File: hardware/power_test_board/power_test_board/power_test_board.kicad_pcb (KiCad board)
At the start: 2 copper layers, 21 parts, among them SW1 YTSC005A0152501B, U1 AXP192

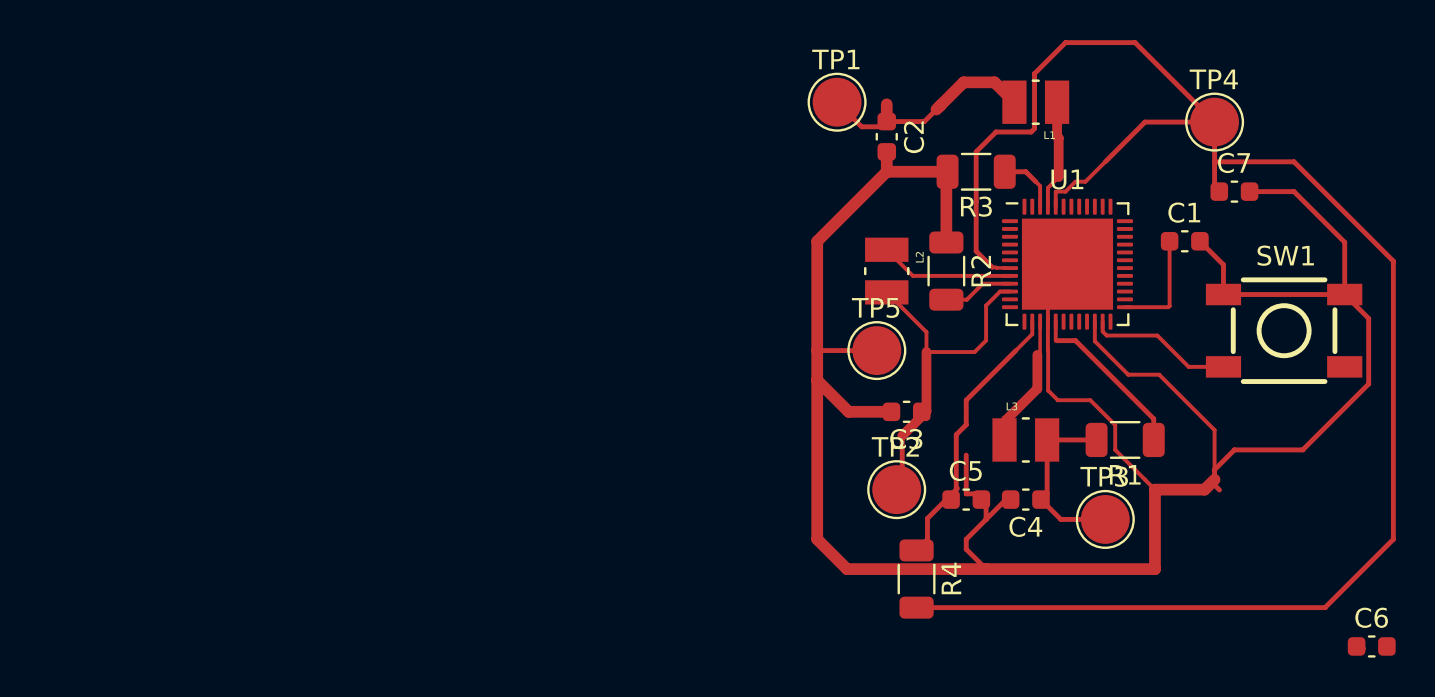
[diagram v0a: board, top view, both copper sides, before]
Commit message: some chnages
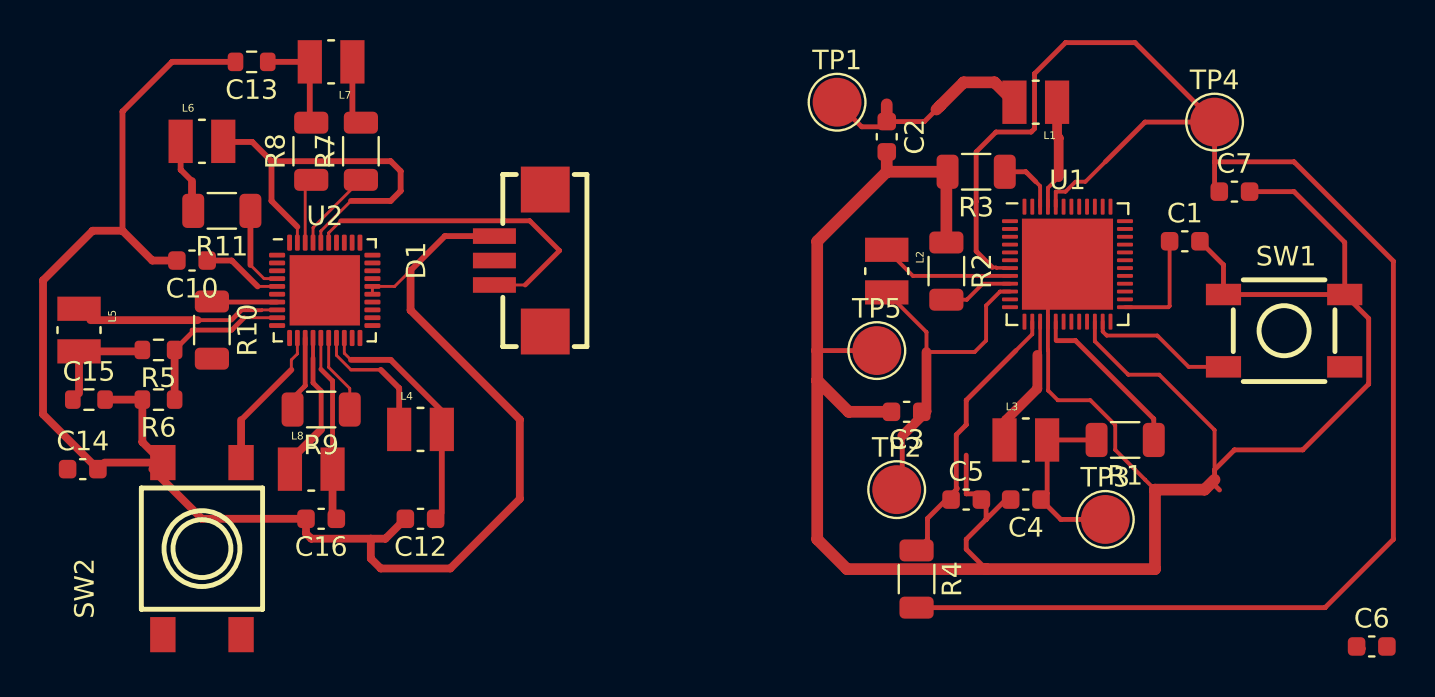
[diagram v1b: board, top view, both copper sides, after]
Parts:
- added C10: 4.7u, rlib_passive:C_0603_1608Metric, F.Cu at (104.7, 82.3)
- added C12: 22u, rlib_passive:C_0603_1608Metric, F.Cu at (116.4, 95.5)
- added C13: 22u, rlib_passive:R_0603_1608Metric, F.Cu at (107.7, 72.1)
- added C14: 22u, rlib_passive:C_0603_1608Metric, F.Cu at (99.1, 92.9)
- added C15: 10u, rlib_passive:R_0603_1608Metric, F.Cu at (99.4, 89.4)
- added C16: 22u, rlib_passive:C_0603_1608Metric, F.Cu at (111.3, 95.5)
- added D1: HCTL HC-1.25-3PWT, rlib_connectors:CONN-SMD_HC-1.25-3PWT, F.Cu at (121.4, 82.3)
- added L4: 2.2u, rlib_passive:INDC2520X120N, F.Cu at (116.4, 90.9)
- added L5: 2.2u, rlib_passive:INDC2520X120N, F.Cu at (98.9, 85.8)
- added L6: 2.2u, rlib_passive:INDC2520X120N, F.Cu at (105.2, 76.2)
- added L7: 2.2u, rlib_passive:INDC2520X120N, F.Cu at (111.8, 72.1)
- added L8: 2.2u, rlib_passive:INDC2520X120N, F.Cu at (110.8, 92.9)
- added R10: 0, Resistor_SMD:R_1206_3216Metric, F.Cu at (105.7, 85.8)
- added R11: 0, Resistor_SMD:R_1206_3216Metric, F.Cu at (106.2, 79.7)
- added R5: R, rlib_passive:R_0603_1608Metric, F.Cu at (103.0, 86.8)
- added R6: R, rlib_passive:R_0603_1608Metric, F.Cu at (103.0, 89.4)
- added R7: 0, Resistor_SMD:R_1206_3216Metric, F.Cu at (113.3, 76.7)
- added R8: 0, Resistor_SMD:R_1206_3216Metric, F.Cu at (110.8, 76.7)
- added R9: 0, Resistor_SMD:R_1206_3216Metric, F.Cu at (111.3, 89.9)
- added SW2: K2-1156SP-F5SW-05, rlib_buttons:K2-1156SP-F5SW-05, F.Cu at (105.2, 97.0)
- added U2: RK816, Package_DFN_QFN:QFN-40-1EP_5x5mm_P0.4mm_EP3.6x3.6mm, F.Cu at (111.5, 83.8)
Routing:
- net GND: track 133.7 -> 223.0 mm
- net VCC: track 90.5 -> 115.5 mm
- net Net-(D1-Pad1): track 0.00 -> 17.3 mm
- net +1V1: track 0.00 -> 12.6 mm
- net Net-(L5-Pad1): track 0.00 -> 10.6 mm
- net Net-(U2-Pad15): track 0.00 -> 9.57 mm
- net Net-(R5-Pad1): track 0.00 -> 8.81 mm
- net Net-(SW2-Pad3): track 0.00 -> 7.56 mm
- net Net-(U2-Pad14): track 0.00 -> 7.54 mm
- net Net-(L4-Pad1): track 0.00 -> 6.90 mm
- net +2V5: track 0.00 -> 6.32 mm
- net +3V3: track 0.00 -> 5.29 mm
- net Net-(U2-Pad4): track 0.00 -> 4.42 mm
- net Net-(U2-Pad37): track 0.00 -> 4.23 mm
- net Net-(C10-Pad1): track 0.00 -> 4.12 mm
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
